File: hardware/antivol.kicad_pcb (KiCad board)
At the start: 2 copper layers, 34.2 x 20.3 mm, 38 parts, among them J1 Conn_01x02, J2 Conn_01x06, J3 Conn_01x02, Q1 AO3401A, Q2 AO3401A, Q3 AO3401A, U1 ESP-WROOM-32, U2 TP4054, U3 ME6211C33, U4 KXTJ3-1057

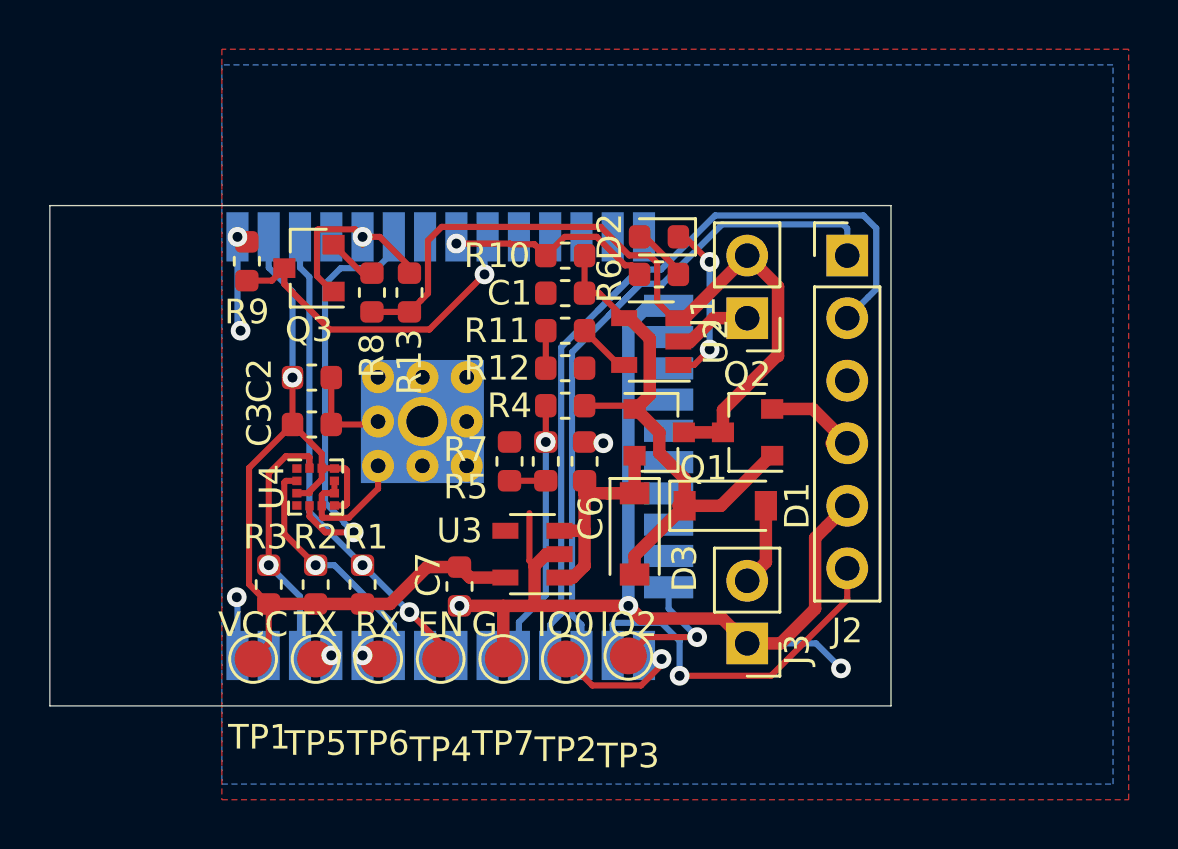
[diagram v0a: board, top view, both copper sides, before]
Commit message: v1
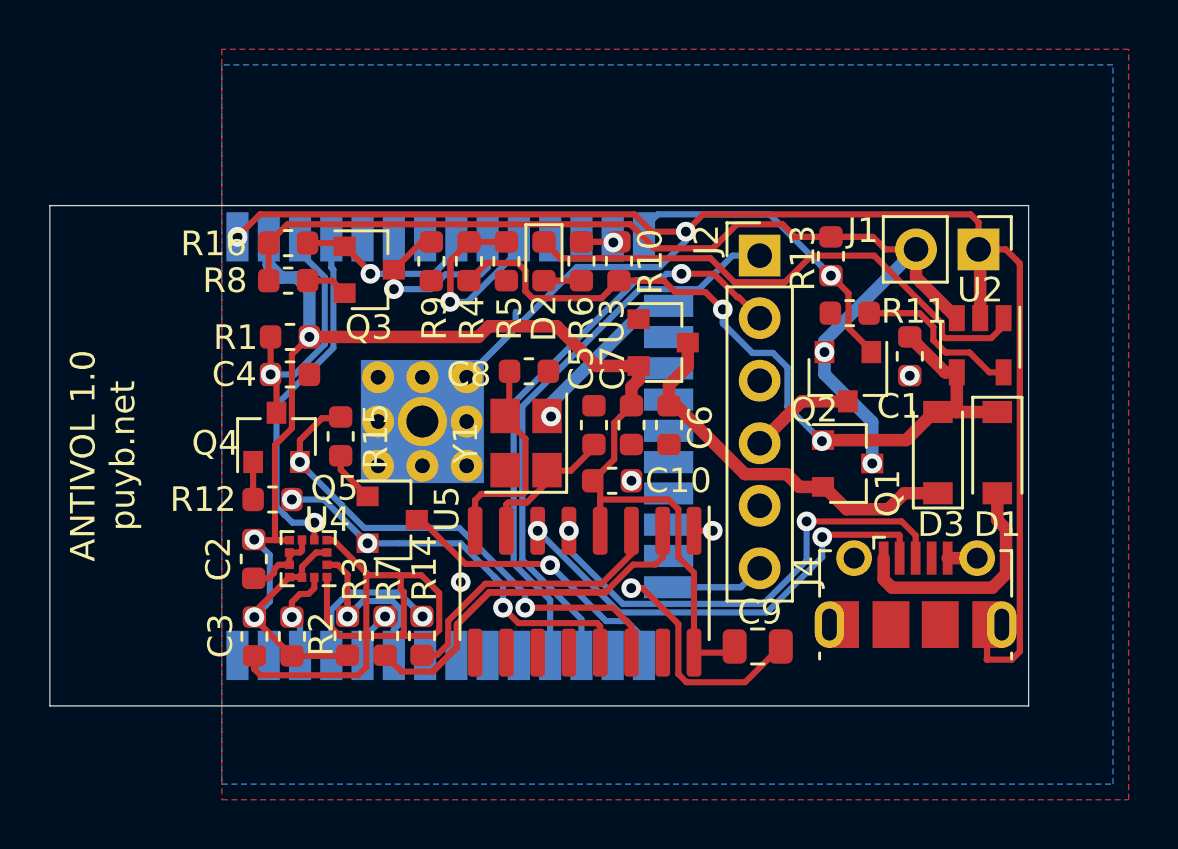
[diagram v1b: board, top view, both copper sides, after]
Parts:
- removed J3: Conn_01x02, Connector_PinHeader_2.54mm:PinHeader_1x02_P2.54mm_Vertical
- removed TP1, TP2, TP3, TP4, TP5, TP6, TP7: TestPoint, TestPoint:TestPoint_Pad_D1.5mm
- added C10: 0.1µF, Capacitor_SMD:C_0603_1608Metric, F.Cu at (66.6, 109.0)
- added C4: 1nF, Capacitor_SMD:C_0603_1608Metric, F.Cu at (53.6, 104.6)
- added C5: 12pF, Capacitor_SMD:C_0603_1608Metric, F.Cu at (65.9, 106.7)
- added C8: 12pF, Capacitor_SMD:C_0603_1608Metric, F.Cu at (63.3, 104.5)
- added C9: 10µF/25V, Capacitor_SMD:C_0805_2012Metric, F.Cu at (72.6, 115.7)
- added J4: USB_B_Micro, Connector_USB:USB_Micro-B_Molex-105017-0001, F.Cu at (79.0, 113.6)
- added Q4: S8050, Package_TO_SOT_SMD:SOT-23, F.Cu at (53.0, 107.2)
- added Q5: S8050, Package_TO_SOT_SMD:SOT-23, F.Cu at (57.7, 110.6)
- added R14: 470, Resistor_SMD:R_0603_1608Metric, F.Cu at (58.9, 115.3)
- added R15: 10k, Resistor_SMD:R_0603_1608Metric, F.Cu at (55.6, 107.2)
- added R16: 22k, Resistor_SMD:R_0603_1608Metric, F.Cu at (53.5, 99.3)
- added U5: CH340G, Package_SO:SOIC-16_3.9x9.9mm_P1.27mm, F.Cu at (65.5, 113.5)
- added Y1: 12MHz, Crystal:Crystal_SMD_3225-4Pin_3.2x2.5mm, F.Cu at (63.2, 107.4)
- C2: value 10nF -> 0.1µF
- R1, R11: value 1k -> 2.2k
- R12: value 1k -> 10k
- R13, R5: value 10k -> 22k
- R7: value 10k -> 470
- U3: value ME6211C33 -> XC6206P332; footprint Package_TO_SOT_SMD:SOT-23-5 -> Package_TO_SOT_SMD:SOT-23
- moved R13 17.2 mm to (75.5, 99.8)
- moved C1 14.2 mm to (78.7, 103.9), turned to 270 degrees
- moved U2 13.4 mm to (81.6, 103.5), turned to 270 degrees
- moved R12 13.0 mm to (52.9, 109.7)
- moved D3 12.8 mm to (79.9, 107.8), turned to 90 degrees
- moved R11 11.6 mm to (76.3, 102.2)
- moved D1 11.3 mm to (82.3, 107.8), turned to 270 degrees
- moved R1 10.5 mm to (53.6, 103.1), turned to 0 degrees
- moved U3 10.1 mm to (68.7, 103.4), turned to 0 degrees
- moved J1 9.80 mm to (81.5, 99.6), turned to 270 degrees
- moved C7 9.58 mm to (67.4, 106.7)
- moved C3 8.92 mm to (52.1, 115.3), turned to 90 degrees
- moved R7 8.70 mm to (57.4, 115.3)
- moved R5 8.28 mm to (62.4, 100.1)
- moved Q1 7.76 mm to (76.2, 108.3)
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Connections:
- Q2 pad 1: +5V_USB -> /GSM_PWR
- Q2 pad 2: /GSM_VBAT -> +BATT
- Q2 pad 3: +BATT -> /GSM_VBAT
- R1 pad 1: +3V3 -> /ESP_EN
- R1 pad 2: /ESP_EN -> +3V3
- R11 pad 1: Net-(R11-Pad1) -> GND
- R12 pad 1: GND -> Net-(Q5-Pad2)
- R12 pad 2: Net-(R11-Pad1) -> Net-(Q4-Pad1)
- R13 pad 1: +BATT -> /GSM_PWR
- R13 pad 2: /ADC_EN -> +BATT
- R5 pad 1: Net-(R5-Pad1) -> GND
- R7 pad 1: GND -> /ESP_RX
- R7 pad 2: Net-(R5-Pad1) -> Net-(R7-Pad2)
- U1 pad 10: (no net) -> /USB_PWR
- U1 pad 13: (no net) -> /CHARG
- U1 pad 14: (no net) -> /GSM_PWR
- U1 pad 24: /ESP_IO2 -> /GSM_KEY
- U1 pad 26: /GSM_KEY -> (no net)
- U1 pad 29: /USB_PWR -> (no net)
- U1 pad 4: (no net) -> /ACCEL_INT
- U1 pad 5: /ADC_EN -> (no net)
- U1 pad 6: /ACCEL_INT -> (no net)
- U1 pad 8: /CHARG -> /ADC_EN
- U3 pad 1: Net-(C6-Pad1) -> GND
- U3 pad 2: GND -> +3V3
- U4 pad 1: (no net) -> GND
- U4 pad 4: (no net) -> GND
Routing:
- net GND: track 65.1 -> 127.7 mm, vias 7 -> 8
- net +3V3: track 36.7 -> 60.9 mm, vias 1 -> 3
- net Net-(R7-Pad2): track 0.00 -> 24.1 mm
- net Net-(Q4-Pad2): track 0.00 -> 20.6 mm, vias 0 -> 2
- net /USB_D+: track 0.00 -> 19.2 mm, vias 0 -> 2
- net /USB_D-: track 0.00 -> 18.8 mm, vias 0 -> 2
- net Net-(Q5-Pad2): track 0.00 -> 16.6 mm, vias 0 -> 3
- net Net-(D2-Pad1): track 6.88 -> 22.0 mm, vias 2 -> 0
- net /GSM_PWR: track 0.00 -> 13.0 mm, vias 0 -> 1
- net +BATT: track 31.7 -> 43.9 mm, vias 0 -> 2
- net Net-(R14-Pad2): track 0.00 -> 11.7 mm
- net /GSM_KEY: track 15.2 -> 4.17 mm, vias 1 -> 0
- net /GSM_RX: track 34.4 -> 23.8 mm
- net /ESP_EN: track 21.3 -> 11.4 mm, vias 2 -> 1
- net +5V_USB: track 22.9 -> 31.7 mm, vias 0 -> 2
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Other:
- board size 34.2 x 20.3 mm -> 39.8 x 20.3 mm
- board text added: "ANTIVOL 1.0 puyb.net"
- board text removed: "EN"
- board text removed: "G"
- board text removed: "IO0"
- board text removed: "IO2"
- board text removed: "RX"
- board text removed: "TX"
- board text removed: "VCC"
